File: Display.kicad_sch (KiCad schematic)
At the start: 10 parts, among them J3 541043431, U6 1SS383TE85L_F

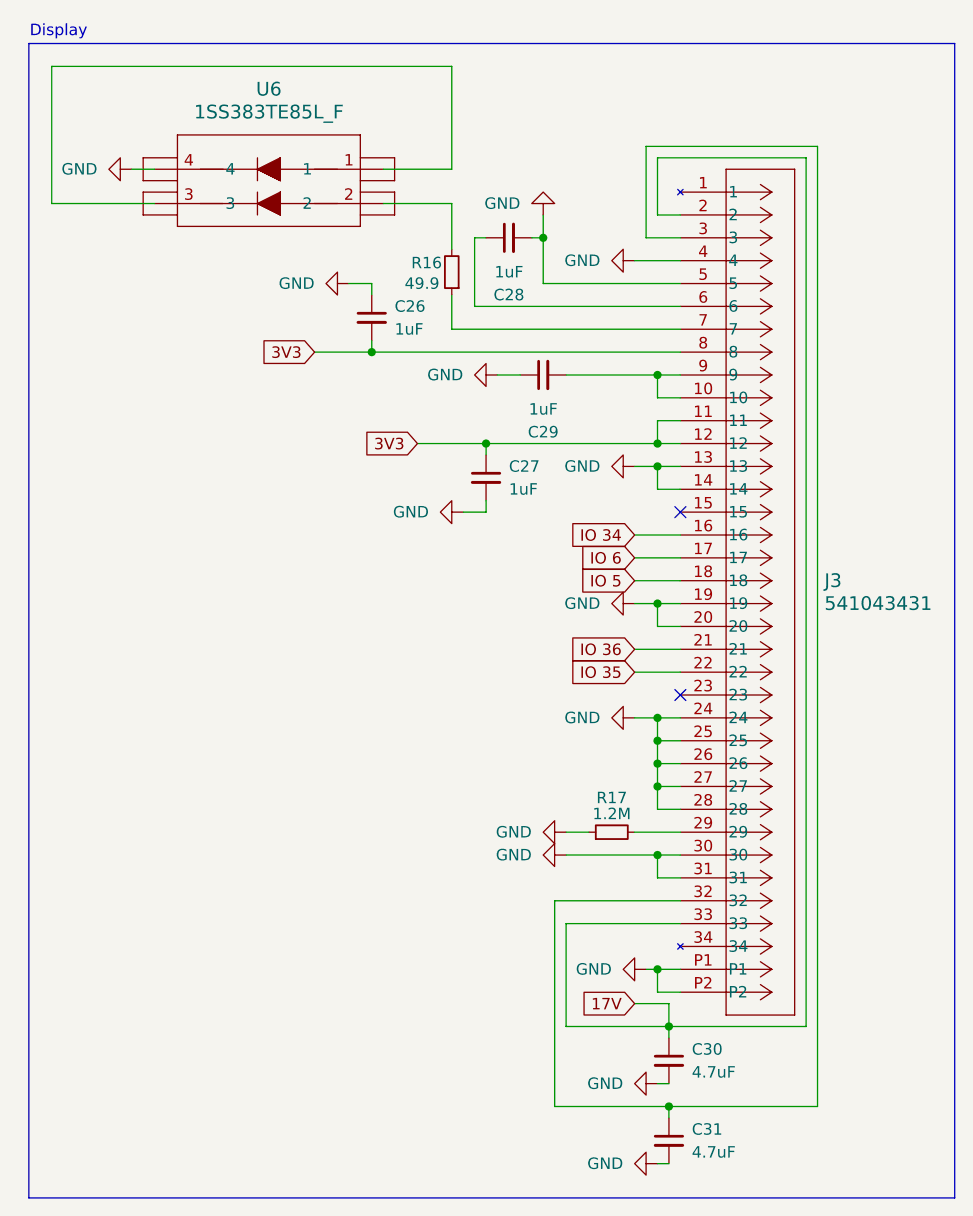
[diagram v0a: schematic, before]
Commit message: Create PCB
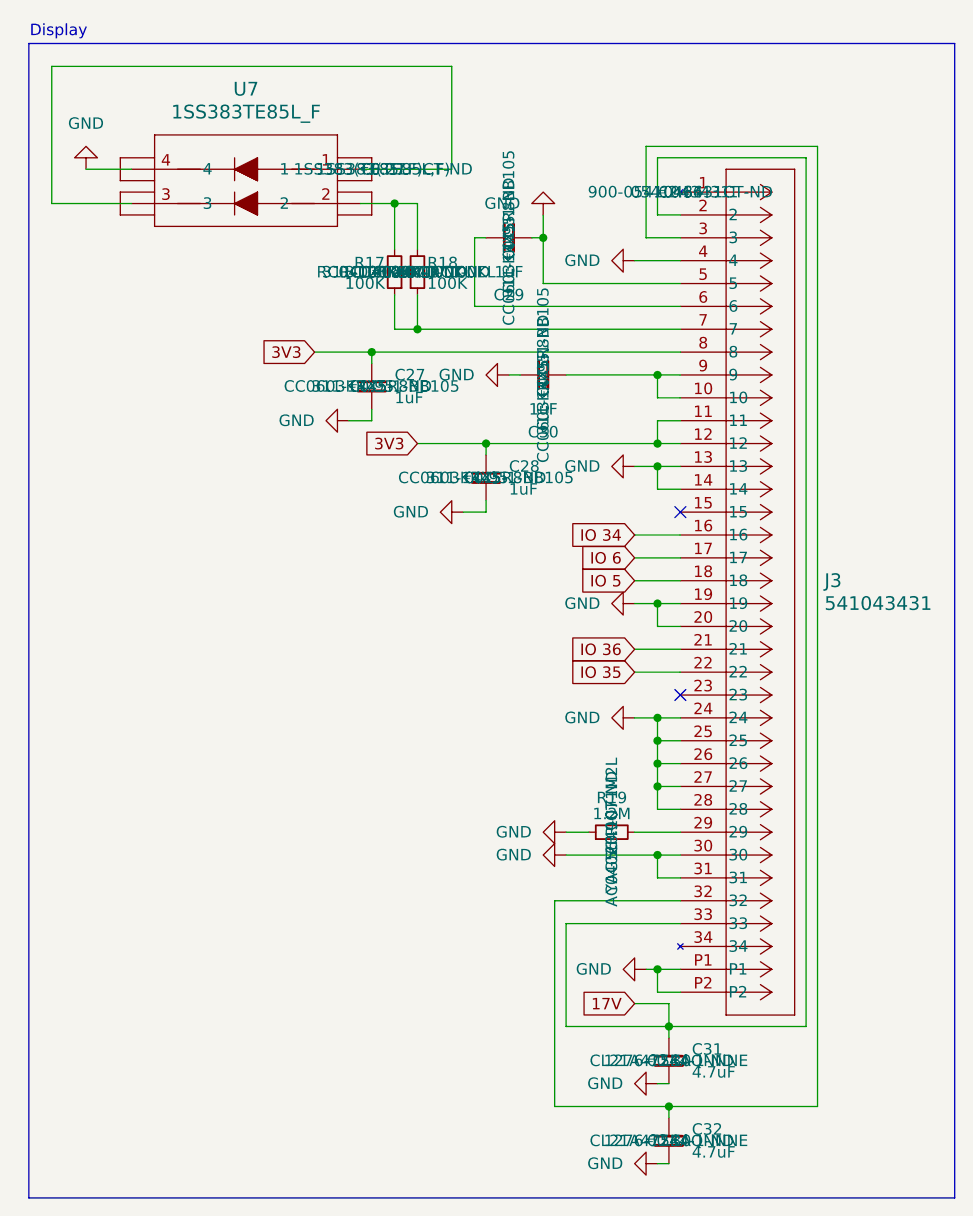
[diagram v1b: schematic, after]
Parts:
- removed C27: 1uF, Capacitor_SMD:C_0603_1608Metric, symbol Device:C_Small
- added C28: 1uF, Capacitor_SMD:C_0603_1608Metric, symbol Device:C_Small
- added R17: 100K, Resistor_SMD:R_0402_1005Metric, symbol Device:R_Small
- C27: renamed from C26; DigiKey_Part_Number (none) -> 311-1445-1-ND; Manufacturer_Part_Number (none) -> CC0603KRX5R8BB105; Price (none) -> €0.95
- C29: renamed from C28; DigiKey_Part_Number (none) -> 311-1445-1-ND; Manufacturer_Part_Number (none) -> CC0603KRX5R8BB105; Price (none) -> €0.95
- C30: renamed from C29; DigiKey_Part_Number (none) -> 311-1445-1-ND; Manufacturer_Part_Number (none) -> CC0603KRX5R8BB105; Price (none) -> €0.95
- C31: renamed from C30; footprint Capacitor_SMD:C_0603_1608Metric -> Capacitor_SMD:C_0805_2012Metric; DigiKey_Part_Number (none) -> 1276-1244-1-ND; Manufacturer_Part_Number (none) -> CL21A475KAQNNNE; Price (none) -> €0.30
- C32: renamed from C31; footprint Capacitor_SMD:C_0603_1608Metric -> Capacitor_SMD:C_0805_2012Metric; DigiKey_Part_Number (none) -> 1276-1244-1-ND; Manufacturer_Part_Number (none) -> CL21A475KAQNNNE; Price (none) -> €0.30
- J3: DigiKey_Part_Number (none) -> 900-0541043431CT-ND; Manufacturer_Part_Number (none) -> 0541043431; Price (none) -> €2.66
- R18: renamed from R16; value 49.9 -> 100K; footprint Resistor_SMD:R_0603_1608Metric -> Resistor_SMD:R_0402_1005Metric; DigiKey_Part_Number (none) -> 311-100KLRCT-ND; Manufacturer_Part_Number (none) -> RC0402FR-07100KL; Price (none) -> €0.40
- R19: renamed from R17; footprint Resistor_SMD:R_0603_1608Metric -> Resistor_SMD:R_0402_1005Metric; DigiKey_Part_Number (none) -> YAG5649CT-ND; Manufacturer_Part_Number (none) -> AC0402FR-071M2L; Price (none) -> €0.10
- U7: renamed from U6; DigiKey_Part_Number (none) -> 1SS383(TE85LF)CT-ND; Manufacturer_Part_Number (none) -> 1SS383(TE85L,F); Price (none) -> €0.27
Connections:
- net 3V3: now also C27.1, C28.1; no longer C27.2
- net GND: now also C27.2, C28.2; no longer C27.1
- net at J3.7, R18.1: now also R17.1
- net at R18.2, U7.2: now also R17.2
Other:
- moved on the sheet: C27, R18, U7
